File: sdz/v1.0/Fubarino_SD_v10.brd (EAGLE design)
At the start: 71.1 x 25.4 mm, 38 parts, among them IC2 MCP1702T-3302E/MB, J1 MICRO_SD_CARD_SOCKET, J2 M28USEPIN1, J3 M28NOPIN1, J8 USB-5PIN, Q1 8MHz, Q2 32.768 KHz

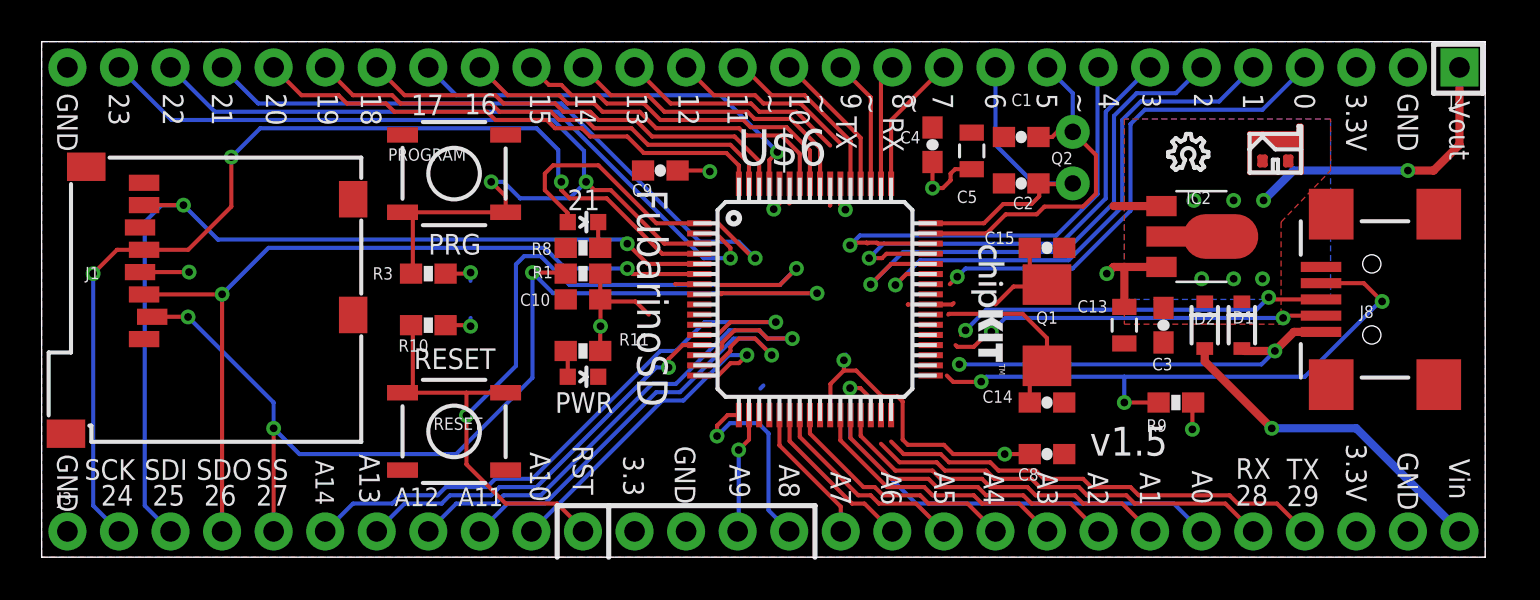
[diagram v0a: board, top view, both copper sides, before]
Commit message: More work on FBSDZ
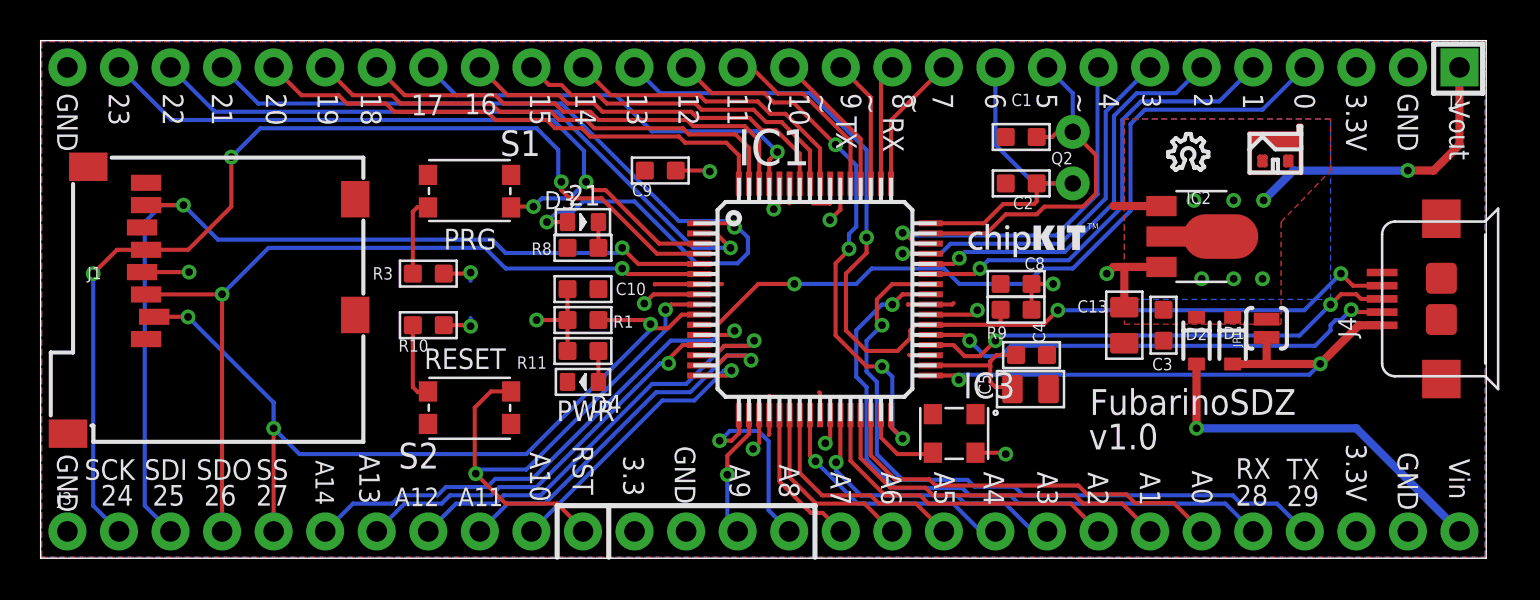
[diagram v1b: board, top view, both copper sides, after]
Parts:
- removed C14, C15: 12pF, SparkFun:0603-CAP
- removed J8: USB-5PIN, SchmalzHaus:USB-MINIB-5PIN-HIROSE-UX60-MB-5ST
- removed LED1: RED, SparkFun:LED-0603
- removed LED2: GREEN, SparkFun:LED-0603
- removed PROGRAM, RESET: PTS525SM10SMTR LFS, SparkFun02-20-08:TACTILE_SWITCH_SMD
- removed Q1: 8MHz, SchmalzHaus:NX5032_5MM_3.2MM_CRYSTAL
- added D3: GREEN, OPL Eagle Library:LED0603
- added D4: RED, OPL Eagle Library:LED0603
- added IC3: DSC1033_MICREL_OSCILLATOR3.2X2.5, SchmalzHaus:3.2X2.5_SILABS_OSC_DSC1033
- added J4: MICRO-USB-5P-340015001, OPL Eagle Library:B-SMD-5P
- added JP1: (no value), SparkFun-Passives:SJ_2S-NO
- added S1, S2: (no value), SchmalzHaus:SWITCH_KMR_SMT_TACT
- C1, C2, C3, C4, C8, C9: device SparkFun:0603-CAP -> OPL Eagle Library:C0603
- C10: device SparkFun02-20-08:0603 -> OPL Eagle Library:C0603
- C13: device SparkFun02-20-08:0805 -> OPL Eagle Library:C0805
- C5: device SchmalzHaus:0805 -> OPL Eagle Library:C0805
- R1, R10, R11, R3, R8, R9: device SparkFun:0603-RES -> OPL Eagle Library:R0603
- moved C5 12.1 mm to (48.7, 8.28), turned to 0 degrees
- moved C4 11.5 mm to (48.8, 9.96), turned to 0 degrees
- moved R9 9.11 mm to (48.0, 12.2)
- moved C8 8.52 mm to (48.0, 13.5), turned to 180 degrees
- moved R1 2.29 mm to (26.7, 11.7), turned to 0 degrees
- moved D1 0.89 mm to (58.7, 10.7)
- moved D2 0.86 mm to (56.9, 10.7)
- moved U$4 0.81 mm to (45.5, 14.7), turned to 0 degrees
- moved C10 0.51 mm to (26.7, 13.2), turned to 0 degrees
- moved J1 0.10 mm to (15.8, 19.7)
- turned R11 to 180 degrees
- renumbered U$6 to IC1
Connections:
- removed net OSC2: C15.2, IC1.32, Q1.2
- removed net RD6: J2.16
- removed net RD7: J2.17
- removed net RD8: J2.4
- removed net USBID: IC1.38, J8.ID, R9.1
- new net RC15: IC1.32, J2.16
- new net USBID/RF3: IC1.38, J2.17, J4.4, R9.1
- net !MCLR!: now also S2.P$3, S2.P$4; no longer RESET.3, RESET.4
- net 3.3V: now also IC3.P$4
- net 5V: now also JP1.2
- net D+: now also J4.3; no longer J8.D+
- net D-: now also J4.2; no longer J8.D-
- net GND: now also D4.-, IC3.P$2, J4.5, J4.E1, J4.E2, J4.P1, J4.P2, S1.P$1, S1.P$2, S2.P$1, S2.P$2; no longer C14.1, C15.1, J8.GND, J8.MTN1, J8.MTN2, J8.MTN3, J8.MTN4, LED1.C, PROGRAM.1, PROGRAM.2, RESET.1, RESET.2
- net N$20: now also D3.-; no longer LED2.C
- net N$6: now also D4.+; no longer LED1.A
- net OSC1: now also IC3.P$3; no longer C14.2, Q1.1
- net RB5: now also J2.4
- net RE5: now also D3.+; no longer LED2.A
- net RE7: now also S1.P$3, S1.P$4; no longer PROGRAM.3, PROGRAM.4
- net VBUS: now also J4.1, JP1.1; no longer J8.VBUS
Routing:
- net USBID/RF3: track 0.00 -> 52.1 mm, vias 0 -> 3
- net RB5: track 0.00 -> 38.2 mm, vias 0 -> 1
- net USBID: track 29.6 -> 0.00 mm, vias 3 -> 0
- net RC15: track 0.00 -> 27.5 mm, vias 0 -> 4
- net RD8: track 24.4 -> 0.00 mm, vias 1 -> 0
- net !MCLR!: track 46.9 -> 30.9 mm
- net RG9: track 55.2 -> 41.3 mm, vias 4 -> 3
- net RF5: track 22.2 -> 33.9 mm, vias 0 -> 1
- net RF4: track 20.1 -> 31.5 mm, vias 0 -> 1
- net RD7: track 11.2 -> 0.00 mm
- net RD6: track 9.15 -> 0.00 mm
- net VBUS: track 20.2 -> 29.1 mm
- net RE7: track 48.3 -> 41.1 mm
- net GND: track 7.91 -> 14.9 mm
- net RD10: track 26.7 -> 20.0 mm
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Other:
- board size 71.1 x 25.4 mm -> 71.2 x 25.5 mm
- board text added: "FubarinoSDZ"
- board text added: "v1.0"
- board text removed: "FubarinoSD"
- board text removed: "v1.5"
